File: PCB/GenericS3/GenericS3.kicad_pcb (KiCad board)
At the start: 2 copper layers, 70 x 70 mm, 71 parts, among them J1 USB-C, J2 Shelly, J3 POWER, P1 33, P10 42, P11 45, P12 46, P13 47, P14 48, P15 18, P16 19, P17 14, P18 15, P19 16, P2 34, P20 17, P21 6, P22 7, P23 8, P24 9, P25 20, P26 10, P27 11, P28 12, P29 13, P3 35, P30 1, P31 2, P32 3, P33 4, P34 5, P35 21, P36 43, P37 44, P38 0, P39 ⏚, P4 36, P40 ⏚, P41 ⏚, P42 ⏚, P43 +, P44 +, P45 +, P46 +, P5 37, P6 38, P7 39, P8 40, P9 41, U1 Barcode, U2 ESP32-S3-MINI-1, U5 MD8942

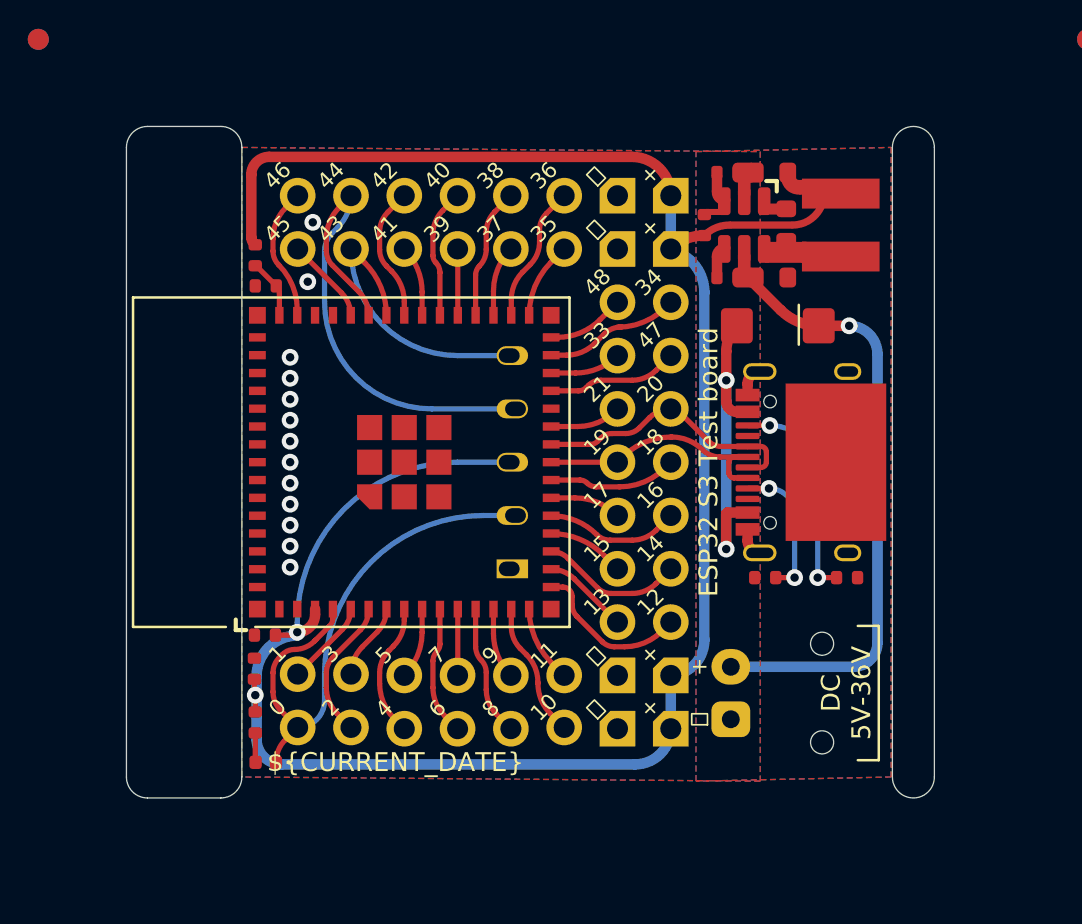
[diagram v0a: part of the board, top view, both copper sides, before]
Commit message: Tweak
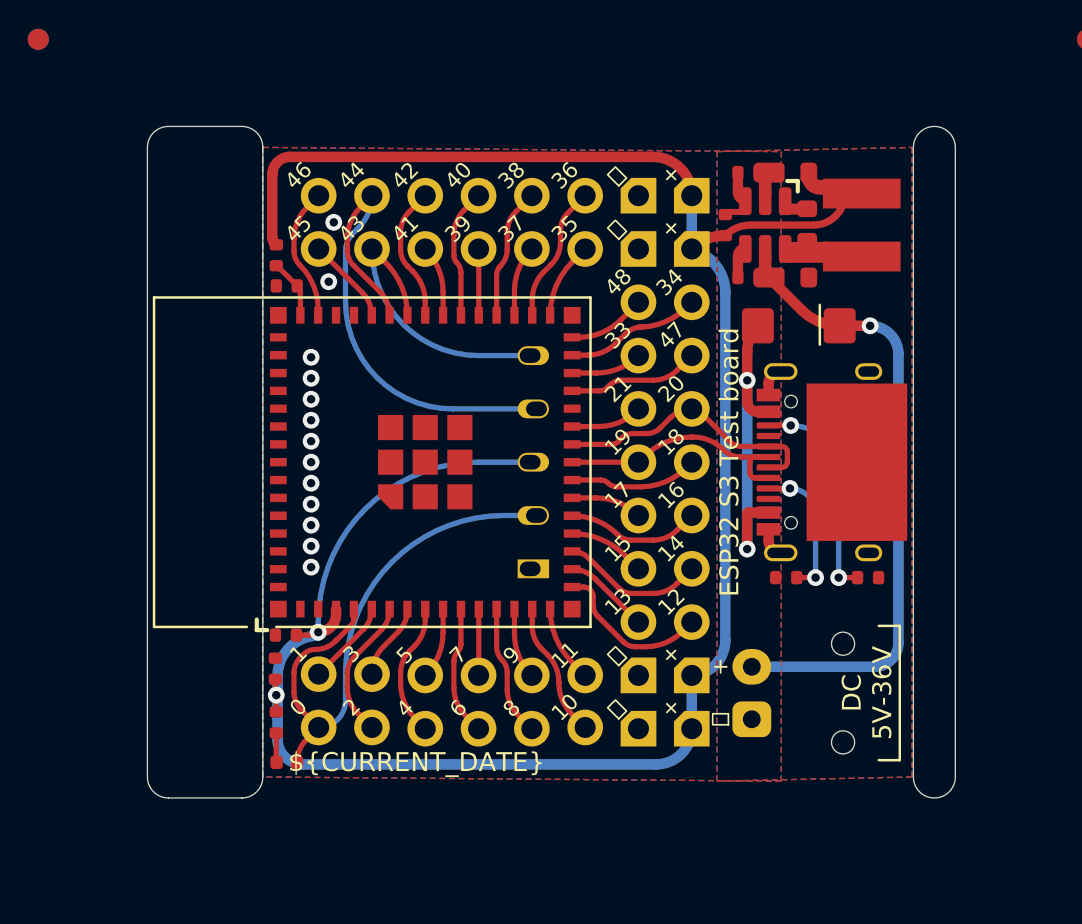
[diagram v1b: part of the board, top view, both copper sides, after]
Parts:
- moved C1 1.00 mm to (86.8, 97.2)
- moved C2 1.00 mm to (86.3, 98.8)
- moved C3 1.00 mm to (86.8, 80.6)
- moved C6 1.00 mm to (110.9, 80.2)
- moved C7 1.00 mm to (110.9, 75.2)
- moved C8 1.00 mm to (111.6, 77.7)
- moved D1 1.00 mm to (111.2, 82.5)
- moved D2 1.00 mm to (86.8, 103.3)
- moved J1 1.00 mm to (112.3, 89.0)
- moved J2 1.00 mm to (98.6, 89.0)
- moved J3 1.00 mm to (109.0, 100.0)
- moved L2 1.00 mm to (114.2, 77.7)
- moved P1 1.00 mm to (103.6, 83.9)
- moved P10 1.00 mm to (93.4, 76.3)
- moved P11 1.00 mm to (88.4, 78.8)
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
